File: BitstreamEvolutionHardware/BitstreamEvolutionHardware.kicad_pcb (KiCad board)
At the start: 2 copper layers, 127 x 106.7 mm, 36 parts, among them J10 61300211121, J11 61300211121, J12 61300211121, J13 61300211121, J14 61300211121, J15 61300211121, J16 61300211121, J17 61300211121, J18 61300211121, J19 61300211121, J20 61300211121, J21 61300211121, J22 61300211121, J23 61300211121, J24 61300211121, J25 61300211121, J26 61300211121, J27 61300211121, J28 61300211121, J29 61300211121, J3 61300211121, J30 61300211121, J31 61300211121, J32 61300211121, J33 61300211121, J34 61300211121, J4 61300211121, J5 61300211121, J6 61300211121, J7 61300211121, J8 61300211121, J9 61300211121, U1 ADS7828, U2 ADS7828, U3 PPTC151LFBN-RC, U4 PPTC151LFBN-RC

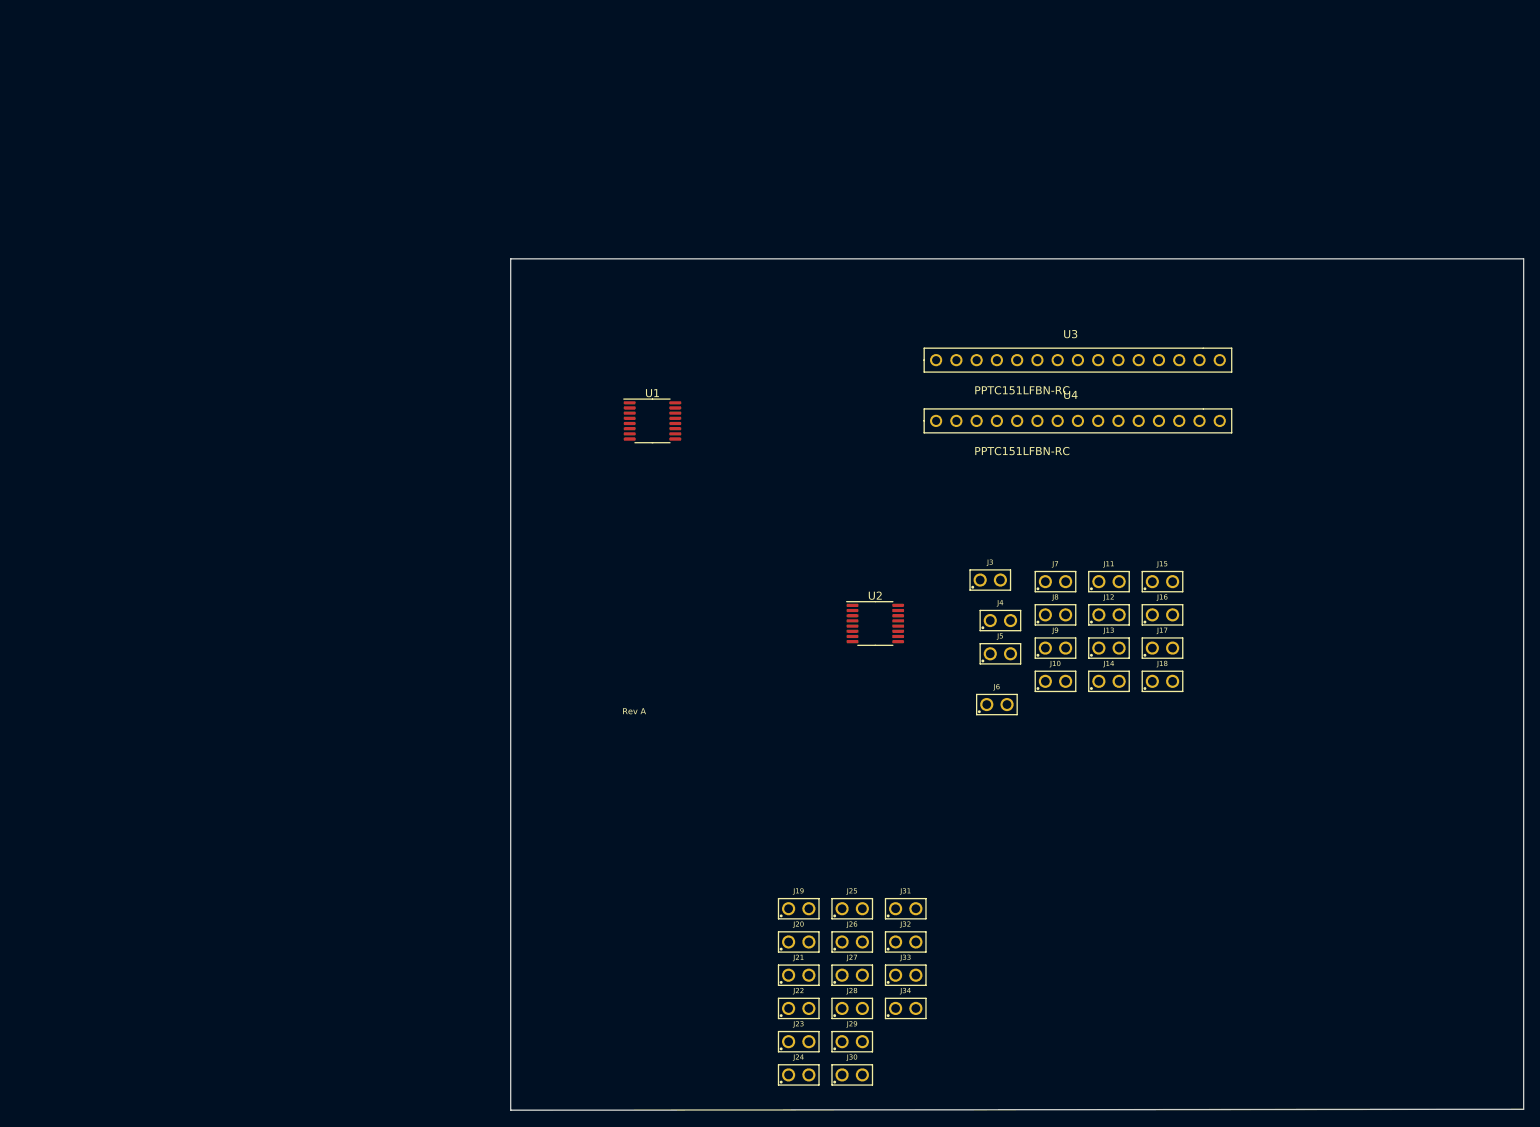
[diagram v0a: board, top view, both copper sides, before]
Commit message: Rev 0.1 Rough Draft Done
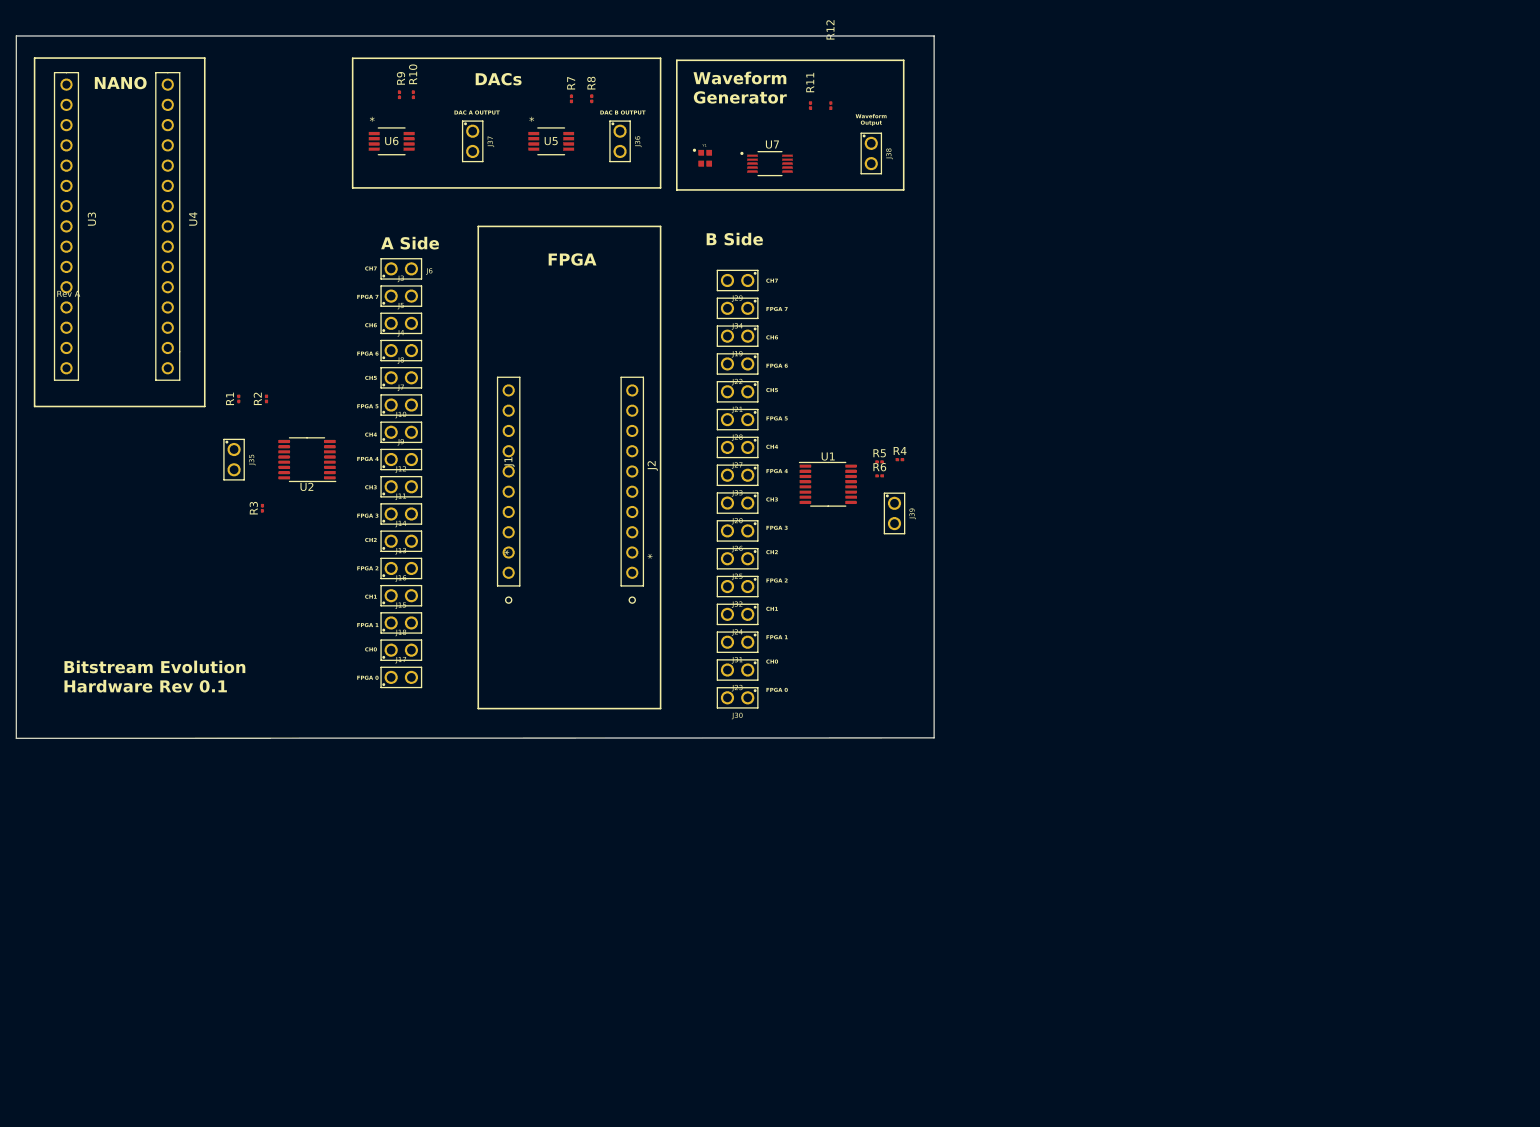
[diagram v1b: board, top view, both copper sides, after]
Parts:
- added J1: PPPC101LFBN-RC, footprints:PPPC101LFBN-RC, F.Cu at (96.3, 87.6)
- added J2: PPPC101LFBN-RC, footprints:PPPC101LFBN-RC, F.Cu at (111.8, 87.6)
- added J35: 61300211121, footprints:61300211121, F.Cu at (61.8, 73.4)
- added J36: 61300211121, footprints:61300211121, F.Cu at (110.2, 33.5)
- added J37: 61300211121, footprints:61300211121, F.Cu at (91.8, 33.5)
- added J38: 61300211121, footprints:61300211121, F.Cu at (141.7, 35.1)
- added J39: 61300211121, footprints:61300211121, F.Cu at (144.6, 80.2)
- added R1: 2K, Resistor_SMD:R_0201_0603Metric, F.Cu at (62.4, 65.8)
- added R10: 2K, Resistor_SMD:R_0201_0603Metric, F.Cu at (84.3, 27.7)
- added R11: 2K, Resistor_SMD:R_0201_0603Metric, F.Cu at (134.1, 29.0)
- added R12: 2K, Resistor_SMD:R_0201_0603Metric, F.Cu at (136.7, 29.0)
- added R2: 2K, Resistor_SMD:R_0201_0603Metric, F.Cu at (65.9, 65.8)
- added R3: 5K, Resistor_SMD:R_0201_0603Metric, F.Cu at (65.4, 79.5)
- added R4: 5K, Resistor_SMD:R_0201_0603Metric, F.Cu at (145.3, 73.4)
- added R5: 2K, Resistor_SMD:R_0201_0603Metric, F.Cu at (142.8, 73.7)
- added R6: 2K, Resistor_SMD:R_0201_0603Metric, F.Cu at (142.8, 75.5)
- added R7: 2K, Resistor_SMD:R_0201_0603Metric, F.Cu at (104.1, 28.2)
- added R8: 2K, Resistor_SMD:R_0201_0603Metric, F.Cu at (106.7, 28.2)
- added R9: 2K, Resistor_SMD:R_0201_0603Metric, F.Cu at (82.6, 27.7)
- added U5: MAX5820MEUA+, footprints:MAX5820MEUA&plus_, F.Cu at (101.6, 33.5)
- added U6: MAX5820MEUA+, footprints:MAX5820MEUA&plus_, F.Cu at (81.6, 33.5)
- added U7: AD9833BRMZ, footprints:SOP50P490X110-10N, F.Cu at (129.0, 36.3)
- added Y1: XRCGB25M000F3M04R0, footprints:OSC_XRCGB25M000F3M04R0, F.Cu at (120.9, 35.6)
- moved U3 114.4 mm to (40.8, 26.4), turned to -90 degrees
- moved U4 105.2 mm to (53.5, 26.4), turned to -90 degrees
- moved J29 96.5 mm to (125.0, 51.0), turned to 180 degrees
- moved J15 95.6 mm to (82.8, 93.9)
- moved J18 95.5 mm to (82.8, 97.3)
- moved J17 95.5 mm to (82.8, 100.7)
- moved J16 95.5 mm to (82.8, 90.5)
- moved J6 92.5 mm to (82.8, 49.5)
- moved J14 90.4 mm to (82.8, 83.7)
- moved J34 90.3 mm to (125.0, 54.5), turned to 180 degrees
- moved J12 90.2 mm to (82.8, 76.8)
- moved J13 89.3 mm to (82.8, 87.1)
- moved J11 89.1 mm to (82.8, 80.3)
- moved J10 87.8 mm to (82.8, 70.0)
- moved J8 87.2 mm to (82.8, 63.2)
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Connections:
- U1 pad 10: unconnected-(U1-REF-Pad10) -> /ADC_REF_B
- U1 pad 12: unconnected-(U1-A0-Pad12) -> /Arduino_+3.3V
- U1 pad 13: unconnected-(U1-A1-Pad13) -> /Arduino_+3.3V
- U1 pad 14: unconnected-(U1-SCL-Pad14) -> /Arduino_SCL
- U1 pad 15: unconnected-(U1-SDA-Pad15) -> /Arduino_SDA
- U1 pad 16: unconnected-(U1-VDD-Pad16) -> /Arduino_+3.3V
- U1 pad 9: unconnected-(U1-GND-Pad9) -> GND
- U2 pad 10: unconnected-(U2-REF-Pad10) -> /ADC_REF_A
- U2 pad 12: unconnected-(U2-A0-Pad12) -> GND
- U2 pad 13: unconnected-(U2-A1-Pad13) -> GND
- U2 pad 14: unconnected-(U2-SCL-Pad14) -> /Arduino_SCL
- U2 pad 15: unconnected-(U2-SDA-Pad15) -> /Arduino_SDA
- U2 pad 16: unconnected-(U2-VDD-Pad16) -> /Arduino_+3.3V
- U2 pad 9: unconnected-(U2-GND-Pad9) -> GND
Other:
- board size 127 x 106.7 mm -> 115.1 x 88.1 mm
- board text added: "A Side"
- board text added: "B Side"
- board text added: "Bitstream Evolution Hardware Rev 0.1"
- board text added: "CH0"
- board text added: "CH1"
- board text added: "CH2"
- board text added: "CH3"
- board text added: "CH4"
- board text added: "CH5"
- board text added: "CH6"
- board text added: "CH7"
- board text added: "DAC A OUTPUT"
- board text added: "DAC B OUTPUT"
- board text added: "DACs"
- board text added: "FPGA"
- board text added: "FPGA 0"
- board text added: "FPGA 1"
- board text added: "FPGA 2"
- board text added: "FPGA 3"
- board text added: "FPGA 4"
- board text added: "FPGA 5"
- board text added: "FPGA 6"
- board text added: "FPGA 7"
- board text added: "NANO"
- board text added: "Waveform Generator"
- board text added: "Waveform Output"
